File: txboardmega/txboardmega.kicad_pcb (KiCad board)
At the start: 2 copper layers, 17 parts, among them J1 Power, J10 Switch 2, J11 Switch 3, J12 Switch 4, J13 Switch 5, J14 Switch 6, J15 Encoder, J16 TX Module, J2 Display, J3 Analog 1, J4 Analog 2, J5 Analog 3, J6 Analog 4, J7 Analog 5, J8 Analog 6, J9 Switch 1, U1 ARD_Mega2560_pro

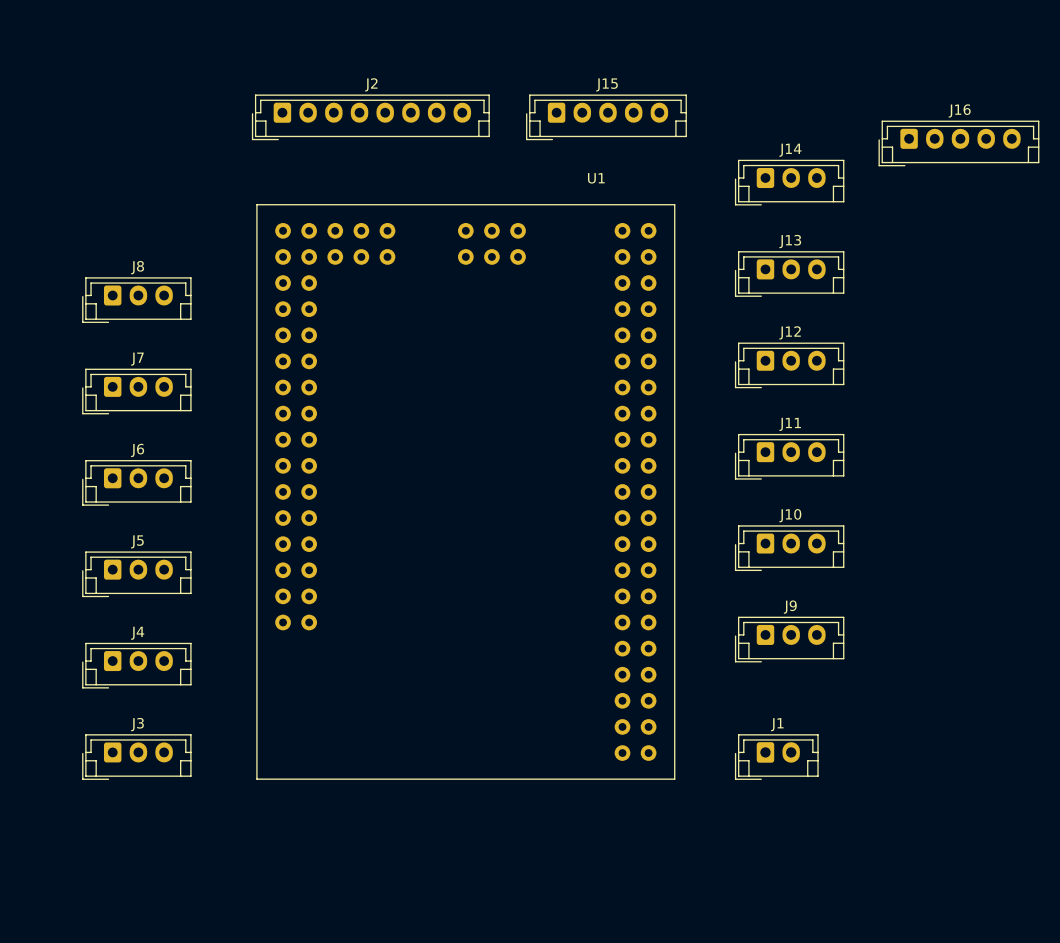
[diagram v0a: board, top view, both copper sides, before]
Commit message: PCB update
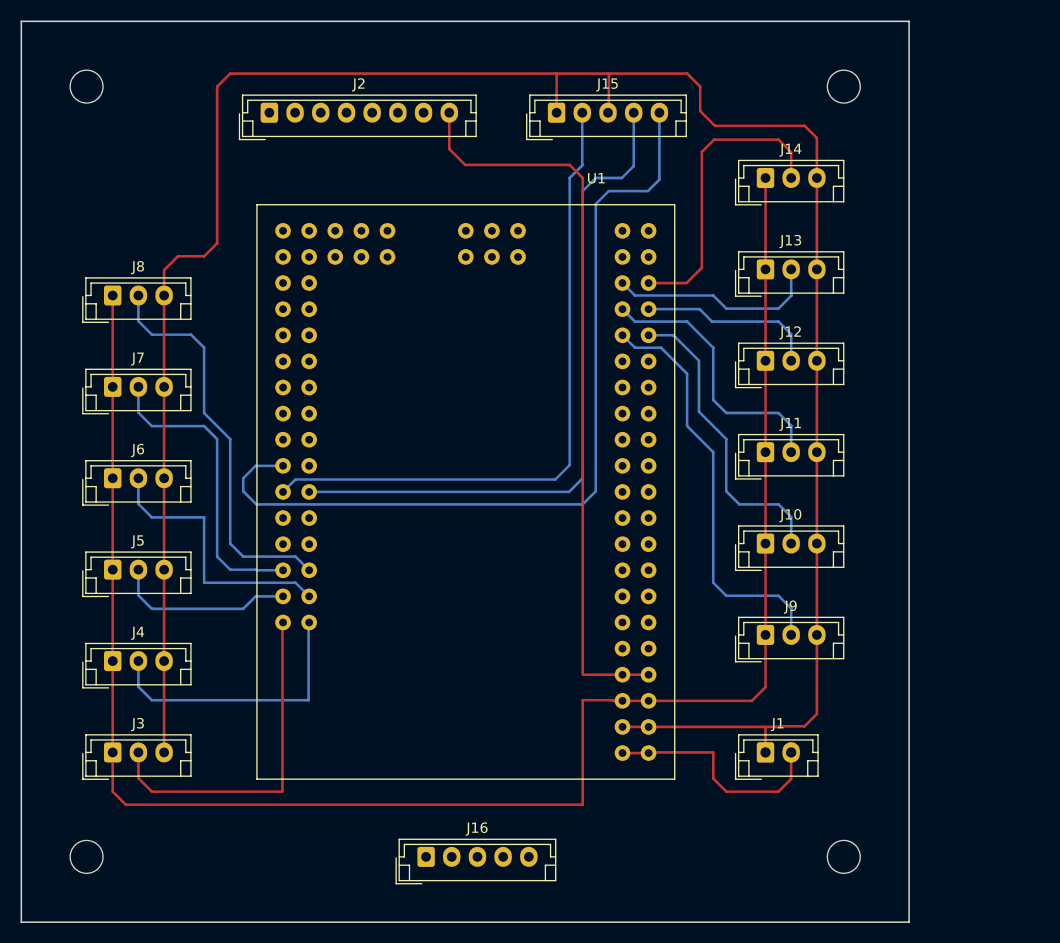
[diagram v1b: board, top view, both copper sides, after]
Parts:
- added REF**: MountingHole_3.2mm_M3_DIN965, MountingHole:MountingHole_3.2mm_M3_DIN965, F.Cu at (174.0, 149.9)
- added REF**: MountingHole_3.2mm_M3_DIN965, MountingHole:MountingHole_3.2mm_M3_DIN965, F.Cu at (100.3, 149.9)
- added REF**: MountingHole_3.2mm_M3_DIN965, MountingHole:MountingHole_3.2mm_M3_DIN965, F.Cu at (174.0, 74.9)
- added REF**: MountingHole_3.2mm_M3_DIN965, MountingHole:MountingHole_3.2mm_M3_DIN965, F.Cu at (100.3, 74.9)
- moved J16 84.2 mm to (133.3, 149.9)
- moved J2 1.27 mm to (118.1, 77.5)
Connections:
- U1 pad 33: Net-(U1-Pad33) -> Net-(J9-Pad2)
- U1 pad 34: Net-(U1-Pad34) -> Net-(J10-Pad2)
- U1 pad 35: Net-(U1-Pad35) -> Net-(J11-Pad2)
- U1 pad 36: Net-(U1-Pad36) -> Net-(J12-Pad2)
- U1 pad 37: Net-(U1-Pad37) -> Net-(J13-Pad2)
- U1 pad 38: Net-(U1-Pad38) -> Net-(J14-Pad2)
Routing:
- net Net-(J1-Pad1): track 0.00 -> 216.9 mm
- net Net-(J10-Pad1): track 0.00 -> 172.6 mm
- net Net-(J15-Pad5): track 0.00 -> 82.6 mm
- net Net-(J2-Pad8): track 0.00 -> 72.3 mm
- net Net-(J15-Pad4): track 0.00 -> 66.3 mm
- net Net-(J15-Pad2): track 0.00 -> 63.8 mm
- net Net-(J9-Pad2): track 0.00 -> 40.4 mm
- net Net-(J8-Pad2): track 0.00 -> 38.8 mm
- net Net-(J3-Pad2): track 0.00 -> 33.5 mm
- net Net-(J10-Pad2): track 0.00 -> 29.7 mm
- net Net-(J7-Pad2): track 0.00 -> 29.6 mm
- net Net-(J14-Pad2): track 0.00 -> 29.3 mm
- net Net-(J4-Pad2): track 0.00 -> 27.2 mm
- net Net-(J11-Pad2): track 0.00 -> 26.7 mm
- net Net-(J6-Pad2): track 0.00 -> 26.6 mm
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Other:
- board outline added: 86.4 x 87.6 mm
